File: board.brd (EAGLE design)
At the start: 74.2 x 27.8 mm, 21 parts, among them U1 FT232RQ

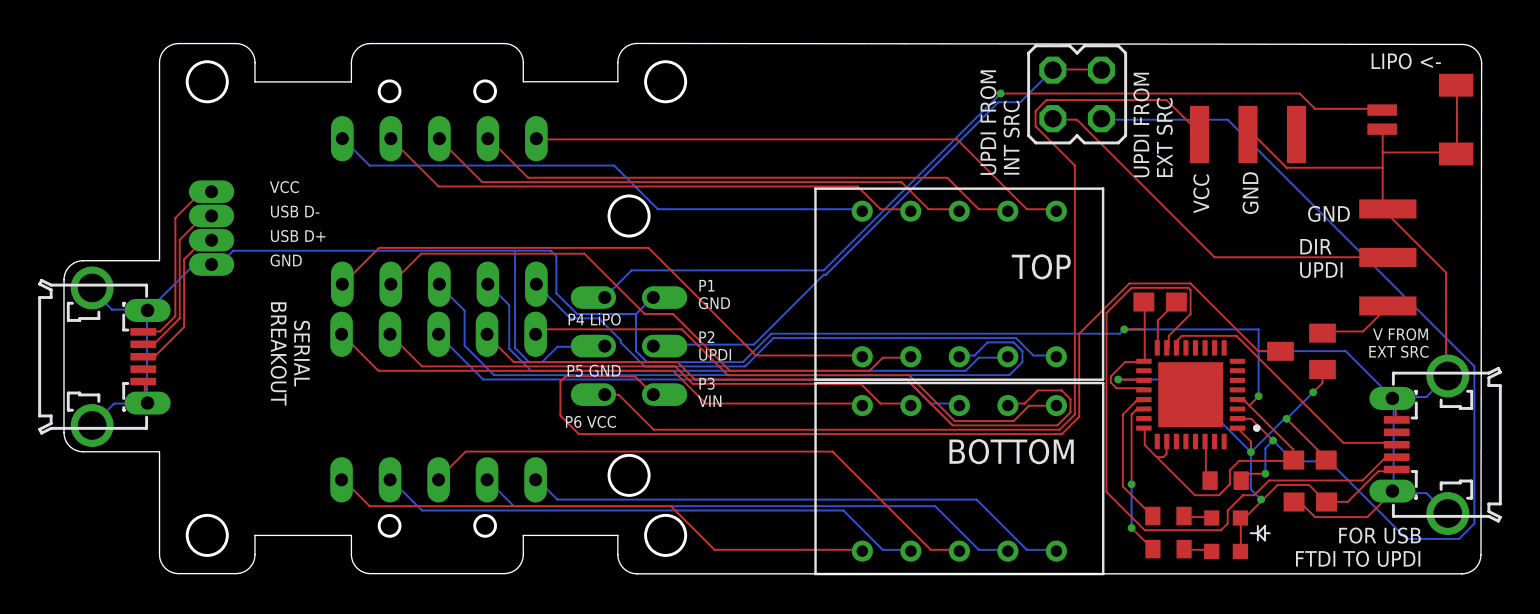
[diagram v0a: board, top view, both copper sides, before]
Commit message: watch file added
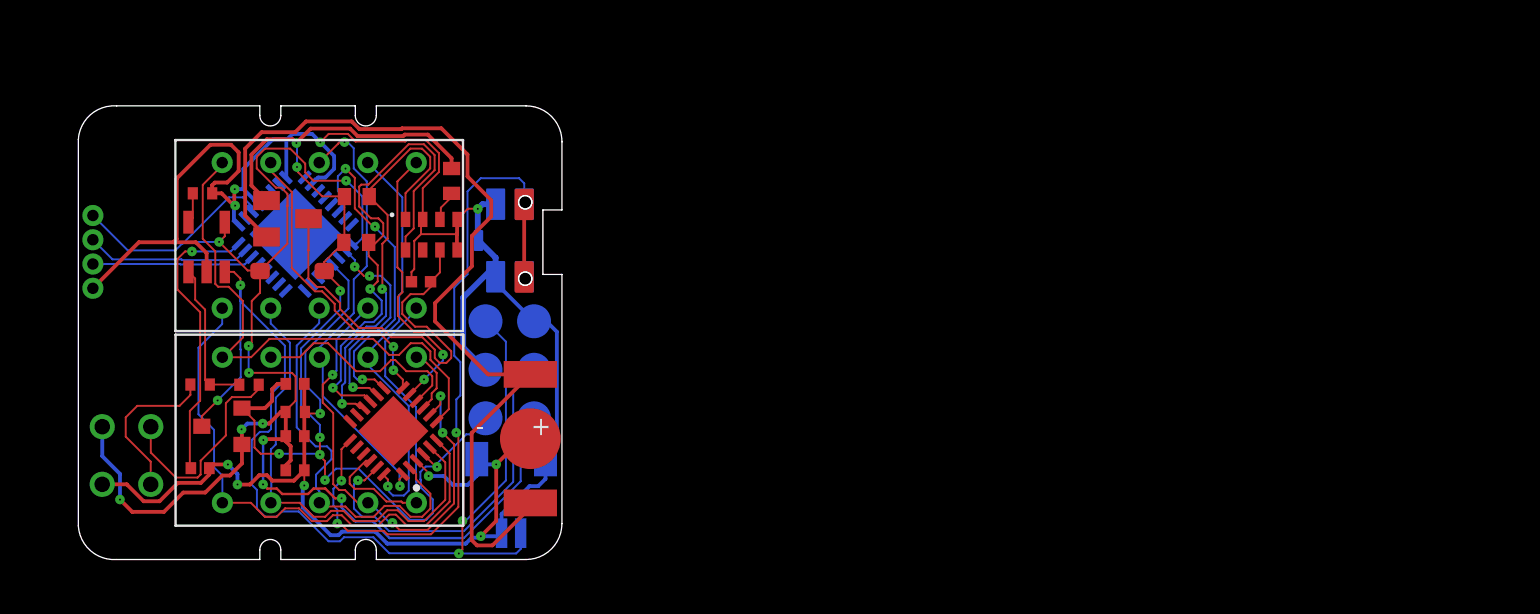
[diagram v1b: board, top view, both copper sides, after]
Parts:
- removed BOTTOM: 0.28"-2DIGIT-7SEGEMNT, MY_CLOCK_LIB_COMPONENTS:2_DIGIT_0.28"
- removed C3: 4.7uF, MY_CLOCK_LIB_COMPONENTS:0603CAP
- removed CLOCK_PCB_TEST_PAD_BREAKOUT, DIRECT_UPDI_PROG_PINS: 3PIN_SMT_MALE, keyboard_lib:3PIN__SMT_MALE
- removed LIPO_BATT_IN_BREAKOUT: JST_SM02B-SRSS-TB, MY_CLOCK_LIB_COMPONENTS:JST-SM02B-SRSS-TB
- removed SERIAL, UPDI: MICROUSB, MY_CLOCK_LIB_COMPONENTS:ZX62D-B-5PA8
- removed U$6: 2X0.28_LED_DISP_POGO_PIN_HARNESS, MY_CLOCK_LIB_COMPONENTS:2X0.28_LED_DISP_POGO_PIN_HARNESS
- removed U1: FT232RQ, FT232RQ:QFN50P500X500X90-33N
- added 1.55V-8MAH: BK-414-TR, MY_CLOCK_LIB_COMPONENTS:BK-414-TR
- added BATTERY_CHARGED_GREEN: GREEN, MY_CLOCK_LIB_COMPONENTS:2MMLED_GREEN
- added BATT_CONNECTED_YELLOW: ORANGE, MY_CLOCK_LIB_COMPONENTS:2MMLED_YELLOW
- added BOT: 0.28"-2DIGIT-7SEGEMNT, MY_CLOCK_LIB_COMPONENTS:2_DIGIT_0.28"
- added C4: 10uF, MY_CAP_LIB:CAPC1005X60
- added C5: 100nF, MY_CAP_LIB:CAPC1005X60
- added C6: 10nF, SparkFun-Capacitors:0402-TIGHT
- added D1: MBR0540, Diodes:SOD-123
- added R4, R5, R7: 4.7K, ARDUINO_3V_TTL_INTERFACE_2_PI:ADAFRUIT_R0402
- added R6: 10K, resistor:RESC1005X40
- added U2: FT232RQ, FT232RQ:QFN50P500X500X90-33N
- added U3: ATTINY1607-MFR, ATTINY1607-MNR:QFN50P400X400X90-25N
- added U4: RV-8803, RV-8803:RV-3028
- added X2: JST_SM02B-SRSS-TB, MY_CLOCK_LIB_COMPONENTS:JST-SM02B-SRSS-TB
- C1: device MY_CLOCK_LIB_COMPONENTS:0603CAP -> MY_CAP_LIB:CAPC1005X60
- C2: value 100nF -> 4.7uF; device MY_CLOCK_LIB_COMPONENTS:0603CAP -> MY_CAP_LIB:CAPC1005X60
- R1, R2: value 270/330 -> 470; device MY_0603_RES:RESC1608X60 -> resistor:RESC1005X40
- R3: value 4.7K -> 10K; device MY_0603_RES:RESC1608X60 -> resistor:RESC1005X40
- U$1: value 2X3-P50-E2-POGOPINS -> MCP73831/2_LIPO_CHARGER; device MY_CLOCK_LIB_COMPONENTS:2X3-P50-E2-POGOPINS -> MY_CLOCK_LIB_COMPONENTS:MCP73831_SOT23-5L
- U$2: value 1X4-1.27-P50-E2-POGOPINS -> 2X3_PAD_ARRAY; device MY_CLOCK_LIB_COMPONENTS:1X4-1.27-P50-E2-POGOPINS -> MY_CLOCK_LIB_COMPONENTS:2X3_PAD_ARRAY
- U$3: value 0603_LED -> DMG341; device MY_CLOCK_LIB_COMPONENTS:0603_LED -> MY_CLOCK_LIB_COMPONENTS:DMG341-P_CHANNEL_MOSFET-SOT23
- U$4: value 0603_LED -> PTS840ESDPMSMTRLF; device MY_CLOCK_LIB_COMPONENTS:0603_LED -> MY_CLOCK_LIB_COMPONENTS:PTS840ESDPMSMTRLF
- U$5: value 2X2PIN_JUMPER -> 4X1.27_FEMALE_EMPTY_CONN; device MY_CLOCK_LIB_COMPONENTS:2X2PIN_JUMPER -> MY_CLOCK_LIB_COMPONENTS:4X1.27_FEMALE_EMPTY_CONN-BACKUP
- moved R3 55.6 mm to (7.25, 19.9)
- moved D2 53.5 mm to (11.7, 18.6), turned to 270 degrees
- moved C2 53.1 mm to (12.1, 7.21), turned to 0 degrees
- moved U$3 52.9 mm to (8.31, 7.72)
- moved U$5 52.5 mm to (1.51, 14.9), turned to 0 degrees
- moved R2 51.2 mm to (7.12, 9.91)
- moved R1 48.9 mm to (9.69, 9.90), turned to 180 degrees
- moved C1 46.1 mm to (12.1, 5.42), turned to 0 degrees
- moved U$4 40.2 mm to (23.3, 17.5), flipped to the bottom, turned to 270 degrees
- moved TOP 33.6 mm to (13.4, 17.7)
- moved U$1 24.0 mm to (7.47, 17.1)
- moved U$2 15.1 mm to (22.1, 13.2), flipped to the bottom, turned to 270 degrees
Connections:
- removed net 3V3OUT: C1.1, U1.16
- removed net B1: BOTTOM._1, U$6.BOT1
- removed net B10: BOTTOM._10, U$6.BOT10
- removed net B2: BOTTOM._2, U$6.BOT2
- removed net B3: BOTTOM._3, U$6.BOT3
- removed net B4: BOTTOM._4, U$6.BOT4
- removed net B5: BOTTOM._5, U$6.BOT5
- removed net B6: BOTTOM._6, U$6.BOT6
- removed net B7: BOTTOM._7, U$6.BOT7
- removed net B8: BOTTOM._8, U$6.BOT8
- removed net B9: BOTTOM._9, U$6.BOT9
- removed net CBUS0: R1.1, U1.22
- removed net CBUS1: R2.1, U1.21
- removed net N$1: R1.2, U$3.C
- removed net SER_USB_DM: SERIAL.2, U$2.P$2
- removed net SER_USB_DP: SERIAL.3, U$2.P$3
- removed net SER_VCC: SERIAL.1, U$2.P$1
- removed net T1: TOP._1, U$6.TOP1
- removed net T10: TOP._10, U$6.TOP10
- removed net T2: TOP._2, U$6.TOP2
- removed net T3: TOP._3, U$6.TOP3
- removed net T4: TOP._4, U$6.TOP4
- removed net T5: TOP._5, U$6.TOP5
- removed net T6: TOP._6, U$6.TOP6
- removed net T7: TOP._7, U$6.TOP7
- removed net T8: TOP._8, U$6.TOP8
- removed net T9: TOP._9, U$6.TOP9
- removed net TXD: R3.1, U1.30
- removed net UPDI_DIR: DIRECT_UPDI_PROG_PINS.2, U$5.4
- removed net UPDI_PROG_DM: U1.15, UPDI.2
- removed net UPDI_PROG_DP: U1.14, UPDI.3
- removed net UPDI_TRANS: R3.2, U$5.2, U1.2
- removed net VIN: D2.3, U$1.6
- removed net V_DIR: D2.2, DIRECT_UPDI_PROG_PINS.1
- new net !INT: R7.2, U4.6
- new net COMM1: TOP._9, U3.12
- new net COMM2: TOP._6, U3.11
- new net COMM3: BOT._9, U3.10
- new net COMM4: BOT._6, U3.9
- new net DOT: BOT._5, TOP._5, U3.22
- new net N$11: C5.1, U2.16
- new net N$4: BATT_CONNECTED_YELLOW.K, R1.1
- new net N$5: R3.1, U$1.5
- new net N$6: BATTERY_CHARGED_GREEN.A, R2.1
- new net RX: U2.2, U3.14
- new net SCL: R4.2, U3.16, U4.8
- new net SDA: R5.2, U3.15, U4.1
- new net SEG_A: BOT._7, TOP._7, U3.24
- new net SEG_B: BOT._8, TOP._8, U3.1
- new net SEG_C: BOT._3, TOP._3, U3.2
- new net SEG_D: BOT._2, TOP._2, U3.5
- new net SEG_E: BOT._1, TOP._1, U3.6
- new net SEG_F: BOT._10, TOP._10, U3.7
- new net SEG_G: BOT._4, TOP._4, U3.8
- new net SW1: U$4.3, U$4.4, U$4.B3, U$4.B4, U3.19
- new net TX: U2.30, U3.13
- new net USBDM: U$5.P$2, U2.15
- new net USBDP: U$5.P$3, U2.14
- new net VBATT: 1.55V-8MAH.1+, 1.55V-8MAH.2+, D2.2
- new net VDD1: C6.1, D2.3, U4.3
- net EXP: now also U2.33; no longer U1.33
- net GND: now also 1.55V-8MAH.-, BATTERY_CHARGED_GREEN.K, C4.2, C5.2, C6.2, R3.2, R6.1, U$2.2, U$2.6, U$4.1, U$4.2, U$4.5, U$5.P$4, U2.17, U2.20, U2.24, U2.26, U2.4, U3.3, U4.4, U4.5, U4.7, X2.1, X2.M1, X2.M2; no longer C3.2, CLOCK_PCB_TEST_PAD_BREAKOUT.2, DIRECT_UPDI_PROG_PINS.3, LIPO_BATT_IN_BREAKOUT.1, LIPO_BATT_IN_BREAKOUT.M1, LIPO_BATT_IN_BREAKOUT.M2, SERIAL.5, SERIAL.S1, SERIAL.S2, SERIAL.S3, SERIAL.S4, U$1.4, U$2.P$4, U1.17, U1.20, U1.24, U1.26, U1.4, UPDI.5, UPDI.S1, UPDI.S2, UPDI.S3, UPDI.S4
- net N$2: now also R1.2, U$1.1; no longer U$4.C
- net UPDI: now also U$2.5, U3.23; no longer U$1.5, U$5.1, U$5.3
- net VCC: now also C4.1, D1.C, D2.1, R4.1, R5.1, R7.1, U$2.3, U$3.2, U3.4; no longer CLOCK_PCB_TEST_PAD_BREAKOUT.3, U$1.3
- net V_LIPO: now also U$1.3, U$2.1, U$3.3, X2.2; no longer LIPO_BATT_IN_BREAKOUT.2, U$1.1
- net V_USB: now also BATT_CONNECTED_YELLOW.A, C1.1, D1.A, R6.2, U$1.4, U$2.4, U$3.1, U$5.P$1, U2.1, U2.19; no longer C3.1, D2.1, U$3.A, U$4.A, U1.1, U1.19, UPDI.1
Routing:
- net VIN: track 52.5 -> 0.00 mm
- net V_USB: track 35.0 -> 87.1 mm, vias 5 -> 10
- net UPDI_TRANS: track 51.8 -> 0.00 mm, vias 2 -> 0
- net VBATT: track 0.00 -> 48.9 mm
- net SW1: track 0.00 -> 41.1 mm, vias 0 -> 3
- net GND: track 176.1 -> 136.6 mm, vias 2 -> 11
- net T3: track 38.3 -> 0.00 mm
- net B7: track 37.3 -> 0.00 mm
- net UPDI_PROG_DM: track 35.9 -> 0.00 mm
- net T4: track 30.7 -> 0.00 mm
- net T2: track 30.7 -> 0.00 mm
- net T1: track 30.4 -> 0.00 mm
- net T5: track 30.1 -> 0.00 mm
- net B3: track 30.1 -> 0.00 mm
- net B6: track 29.7 -> 0.00 mm
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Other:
- board size 74.2 x 27.8 mm -> 25.3 x 23.8 mm
- board text added: "+"
- board text added: "-"
- board text added: "P1"
- board text added: "P2"
- board text added: "P3"
- board text added: "P4"
- board text added: "P5"
- board text added: "P6"
- board text removed: "DIR UPDI"
- board text removed: "FOR USB FTDI TO UPDI"
- board text removed: "GND"
- board text removed: "LIPO <-"
- board text removed: "P1 GND"
- board text removed: "P2 UPDI"
- board text removed: "P3 VIN"
- board text removed: "P4 LiPO"
- board text removed: "P5 GND"
- board text removed: "P6 VCC"
- board text removed: "SERIAL BREAKOUT"
- board text removed: "UPDI FROM EXT SRC"
- board text removed: "UPDI FROM INT SRC"
- board text removed: "V FROM EXT SRC"
- board text removed: "VCC"
- board text removed: "VCC USB D- USB D+ GND"
